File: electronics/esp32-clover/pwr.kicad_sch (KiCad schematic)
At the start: 24 parts, among them Q3 DMG2305UX-13, U3 NCP163ASN330T1G

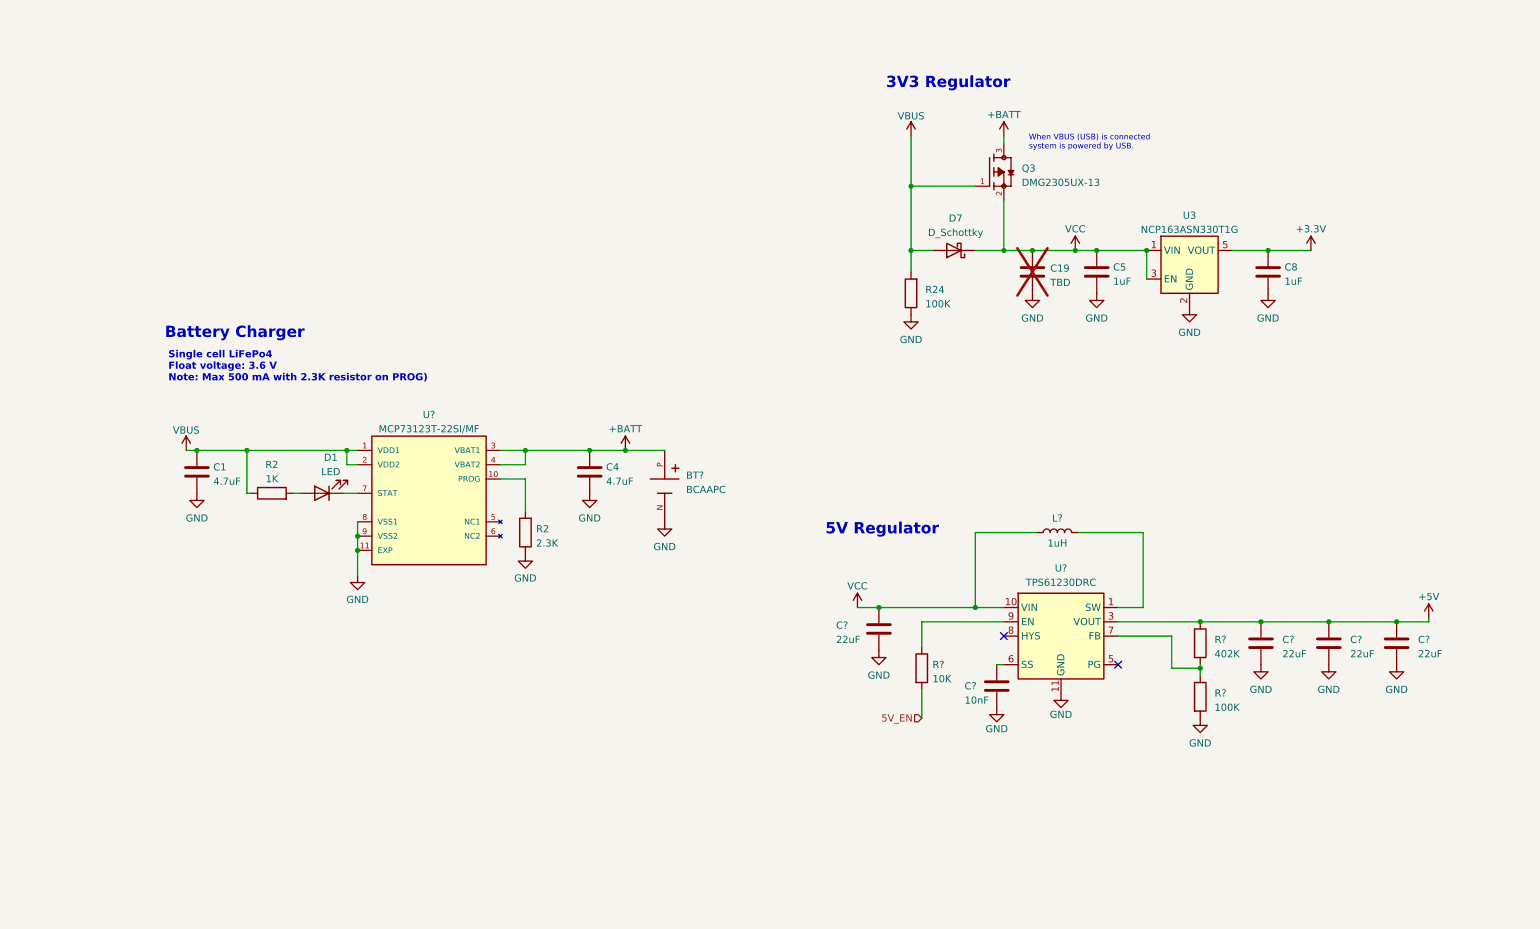
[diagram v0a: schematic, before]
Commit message: update before switching to stm32
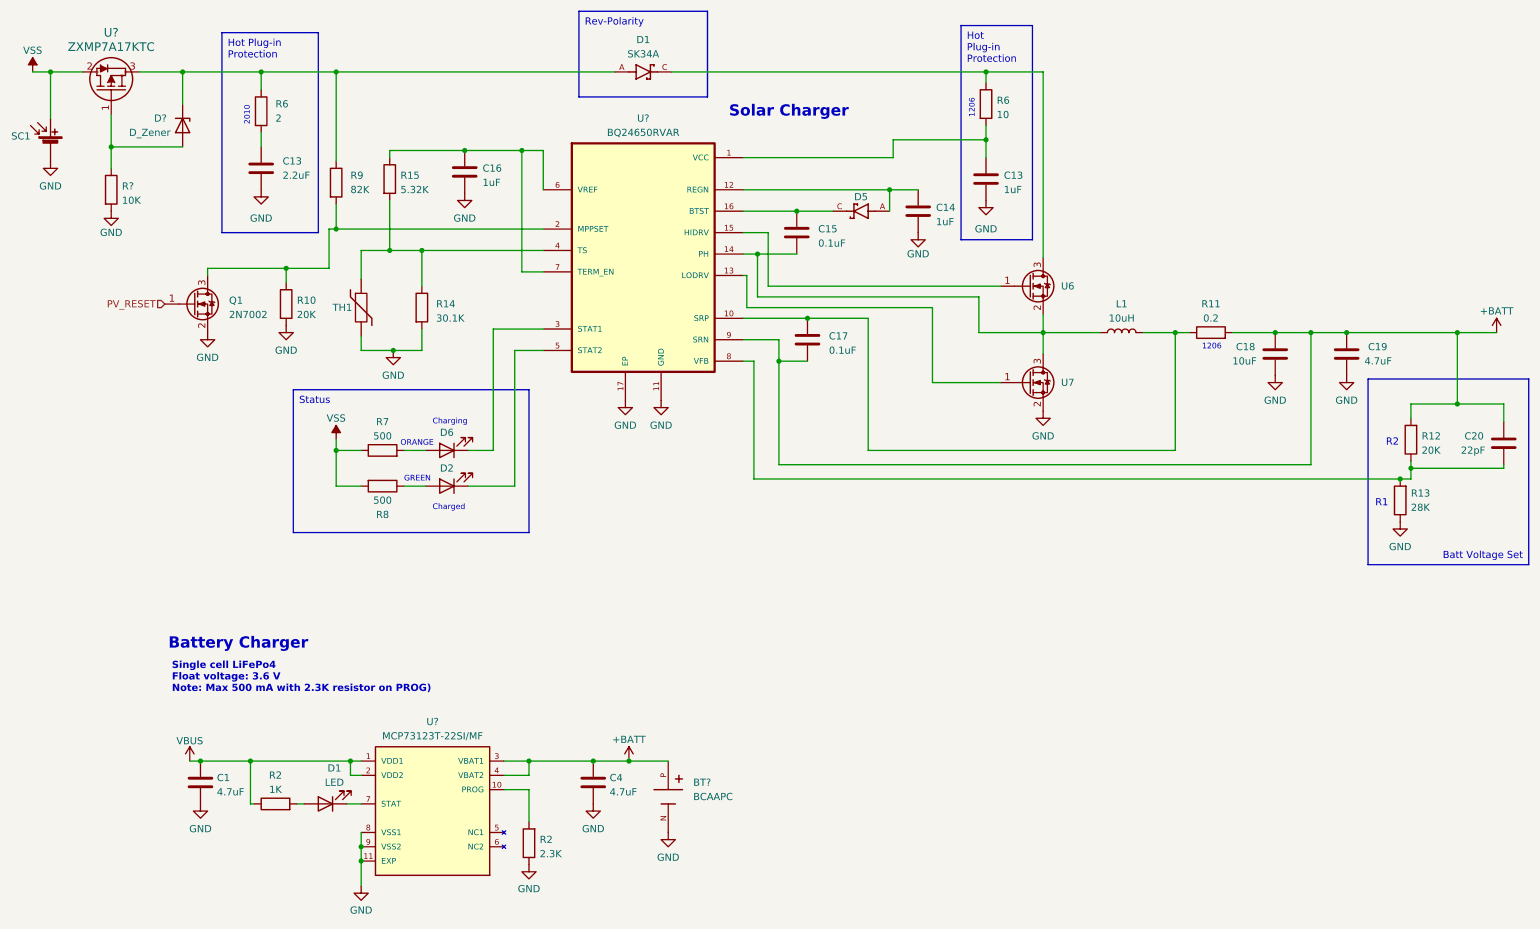
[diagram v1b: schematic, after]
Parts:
- removed BT?: BCAAPC, BAT_BCAAPC, symbol BCAAPC:BCAAPC
- removed C5, C8: 1uF, Capacitor_SMD:C_0603_1608Metric, symbol Device:C
- removed C? (x4): 22uF, symbol Device:C
- removed C?: 10nF, symbol Device:C
- removed D7: D_Schottky, symbol Device:D_Schottky
- removed L?: 1uH, symbol Device:L
- removed Q3: DMG2305UX-13, SOT91P240X110-3N, symbol DMG2305UX-13:DMG2305UX-13
- removed R24: 100K, Resistor_SMD:R_0603_1608Metric, symbol Device:R
- removed R?: 402K, symbol Device:R
- removed R?: 100K, symbol Device:R
- removed R?: 10K, symbol Device:R
- removed U3: NCP163ASN330T1G, Package_TO_SOT_SMD:SOT-23-5, symbol Regulator_Linear:NCP163ASN330T1G
- removed U?: TPS61230DRC, Package_SON:Texas_S-PVSON-N10_ThermalVias, symbol Regulator_Switching:TPS61230DRC
- removed U?: MCP73123T-22SI/MF, SON50P300X300X100-11N, symbol MCP73123T-22SI_MF:MCP73123T-22SI/MF
- added BT?: BCAAPC, battery_holders:BCAAPC, symbol battery_holders:BCAAPC
- added C13: 2.2uF, symbol Device:C
- added C13, C14, C16: 1uF, symbol Device:C
- added C15, C17: 0.1uF, symbol Device:C
- added C18: 10uF, symbol Device:C
- added C20: 22pF, symbol Device:C
- added D1, D5: SK34A, diodes:SK34A, symbol diodes:SK34A
- added D2, D6: LED, symbol Device:LED
- added D?: D_Zener, symbol Device:D_Zener
- added L1: 10uH, symbol Device:L
- added Q1: 2N7002, Package_TO_SOT_SMD:SOT-23, symbol Transistor_FET:2N7002
- added R10, R12: 20K, symbol Device:R
- added R11: 0.2, symbol Device:R
- added R13: 28K, symbol Device:R
- added R14: 30.1K, symbol Device:R
- added R15: 5.32K, symbol Device:R
- added R6: 2, symbol Device:R
- added R6: 10, symbol Device:R
- added R7, R8: 500, symbol Device:R
- added R9: 82K, symbol Device:R
- added R?: 10K, symbol Device:R
- added SC1: Solar_Cell, symbol Device:Solar_Cell
- added TH1: ~, symbol Device:Thermistor
- added U6, U7: PMV30UN, mosfets:PMV30UN, symbol mosfets:PMV30UN
- added U?: ZXMP7A17KTC, mosfets:ZXMP7A17KTC, symbol mosfets:ZXMP7A17KTC
- added U?: BQ24650RVAR, solar_chargers:BQ24650RVAR, symbol solar_chargers:BQ24650RVAR
- added U?: MCP73123T-22SI/MF, battery_chargers:MCP73123T-22SI_MF, symbol battery_chargers:MCP73123T-22SI/MF
- C19: value TBD -> 4.7uF; footprint Capacitor_SMD:C_0603_1608Metric -> (none); now fitted
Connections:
- net VCC is gone; now on net +BATT: C19.1
- net +BATT: now also BT?.P, C17.2, C18.1, C20.1, R11.2, R12.2, U?.3 (VBAT1), U?.4 (VBAT2), U?.9 (SRN)
- net GND: now also BT?.N, C13.2, C13.2, C14.2, C16.2, C18.2, Q1.2 (S), R10.2, R13.1, R14.2, R?.2, SC1.2 (-), TH1.2, U7.2, U?.11 (EXP), U?.11 (GND), U?.17 (EP), U?.8 (VSS1), U?.9 (VSS2)
- net VBUS: now also U?.1 (VDD1), U?.2 (VDD2)
- net at D1.1 (K): now also U?.7 (STAT)
- net at R2.2: now also U?.10 (PROG)
- new net: U7.1, U?.13 (LODRV)
- new net: C15.2, L1.1, U6.2, U7.3, U?.14 (PH)
- new net: C14.1, D5.A, U?.12 (REGN)
- new net: C13.1, R6.2
- new net: D2.1 (K), U?.5 (STAT2)
- new net: D2.2 (A), R8.1
- new net: D?.2 (A), R?.1, U?.1
- new net: Q1.3 (D), R10.1, R9.2, U?.2 (MPPSET)
- new net: C16.1, R15.1, U?.6 (VREF), U?.7 (TERM_EN)
- new net: R14.1, R15.2, TH1.1, U?.4 (TS)
- new net: D1.A, D?.1 (K), R6.1, R9.1, U?.3
- new net: D1.C, R6.1, U6.3
- new net: C17.1, L1.2, R11.1, U?.10 (SRP)
- new net: C13.1, R6.2, U?.1 (VCC)
- new net: C15.1, D5.C, U?.16 (BTST)
- new net: C20.2, R12.1, R13.2, U?.8 (VFB)
- new net: D6.2 (A), R7.2
- new net: U6.1, U?.15 (HIDRV)
- new net: D6.1 (K), U?.3 (STAT1)
- new net PV_RESET: Q1.1 (G)
- new net VSS: R7.1, R8.2, SC1.1 (+), U?.2
- no-connect marks 2 -> 0
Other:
- note added: "1206"
- note added: "2010"
- note added: "Charged"
- note added: "Charging"
- note added: "GREEN"
- note added: "ORANGE"
- note added: "R1"
- note added: "R2"
- note added: "Solar Charger"
- note removed: "3V3 Regulator"
- note removed: "5V Regulator"
- note removed: "When VBUS (USB) is connected system is powered by USB."
- moved on the sheet: C1, C4, D1, R2
